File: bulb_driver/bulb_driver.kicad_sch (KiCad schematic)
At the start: 10 parts, among them J1 Conn_01x02, U1 LM3410DGN, U2 ATtiny13-20S, U3 AP9101CK6

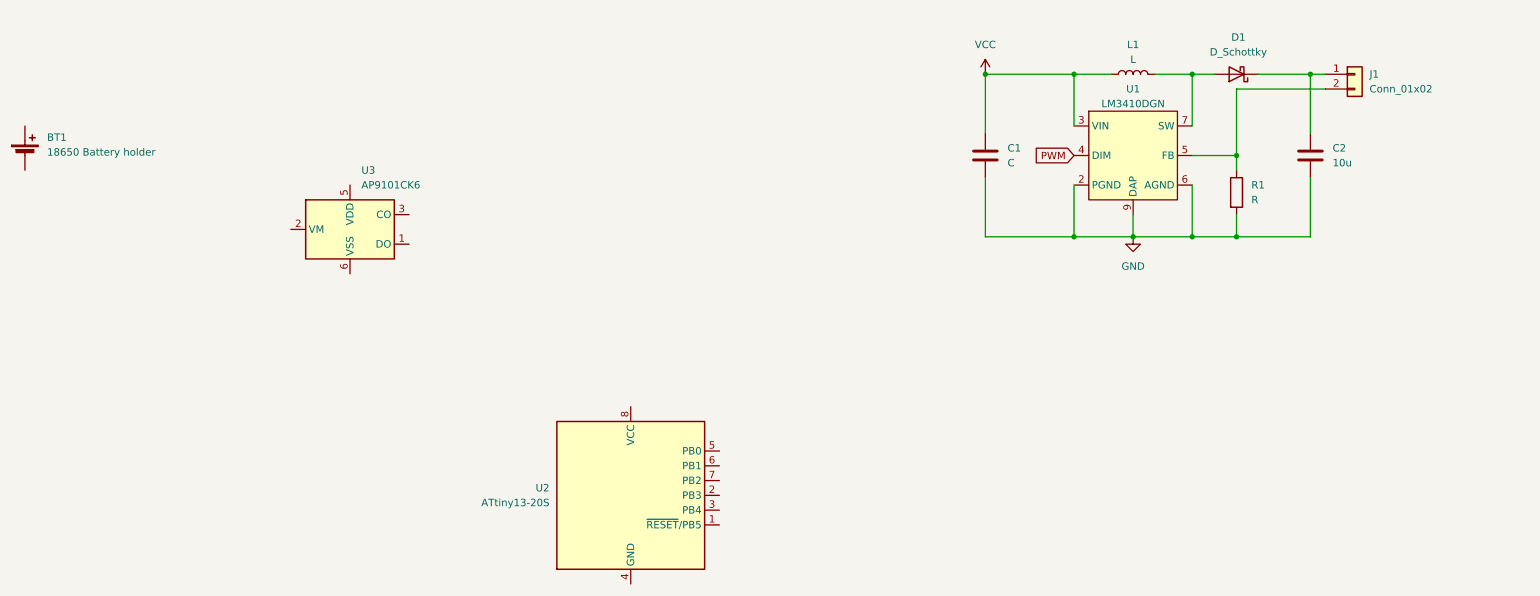
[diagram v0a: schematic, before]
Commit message: Update schematic
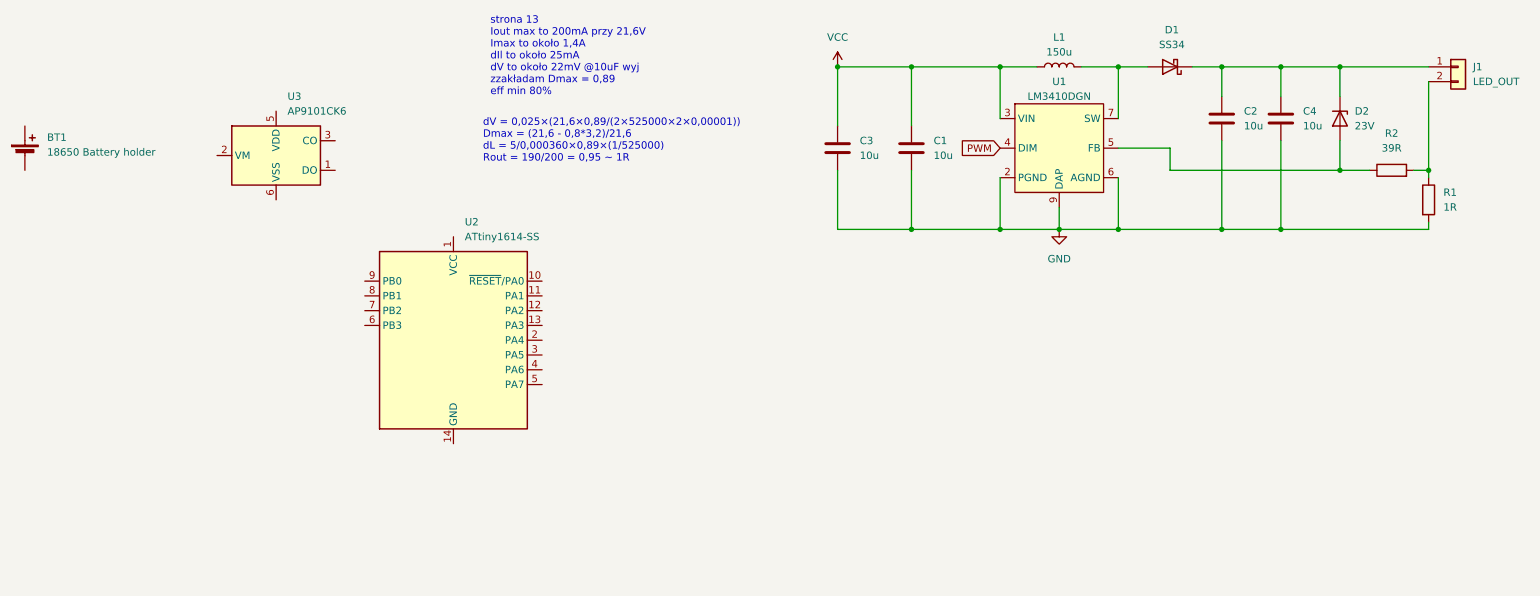
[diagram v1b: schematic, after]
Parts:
- removed U2: ATtiny13-20S, Package_SO:SOIC-8W_5.3x5.3mm_P1.27mm, symbol MCU_Microchip_ATtiny:ATtiny13-20S
- added C3, C4: 10u, symbol Device:C
- added D2: 23V, symbol Device:D_Zener
- added R2: 39R, symbol Device:R
- added U2: ATtiny1614-SS, Package_SO:SOIC-14_3.9x8.7mm_P1.27mm, symbol MCU_Microchip_ATtiny:ATtiny1614-SS
- C1: value C -> 10u
- D1: value D_Schottky -> SS34
- J1: value Conn_01x02 -> LED_OUT
- L1: value L -> 150u
- R1: value R -> 1R
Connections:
- net GND: now also C3.2, C4.2
- net VCC: now also C3.1
- net at J1.2 (Pin_2), R1.1: now also R2.2; no longer U1.5 (FB)
- net at C2.1, D1.1 (K), J1.1 (Pin_1): now also C4.1, D2.1 (K)
- new net: D2.2 (A), R2.1, U1.5 (FB)
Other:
- note added: "dV = 0,025×(21,6×0,89/(2×525000×2×0,00001)) Dmax = (21,6 - 0,8*3,2)/21,6 dL = 5/0,000360×0,89×(1/525000) Rout = 190/200 = 0,95 ~ 1R"
- note added: "strona 13 Iout max to 200mA przy 21,6V Imax to około 1,4A dIl to około 25mA dV to około 22mV @10uF wyj zzakładam Dmax = 0,89 eff min 80%"
- moved on the sheet: C1, C2, D1, J1, L1, R1, U1, U3
